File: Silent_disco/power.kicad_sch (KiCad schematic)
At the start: 1 part, among them J1 USB_B_Micro

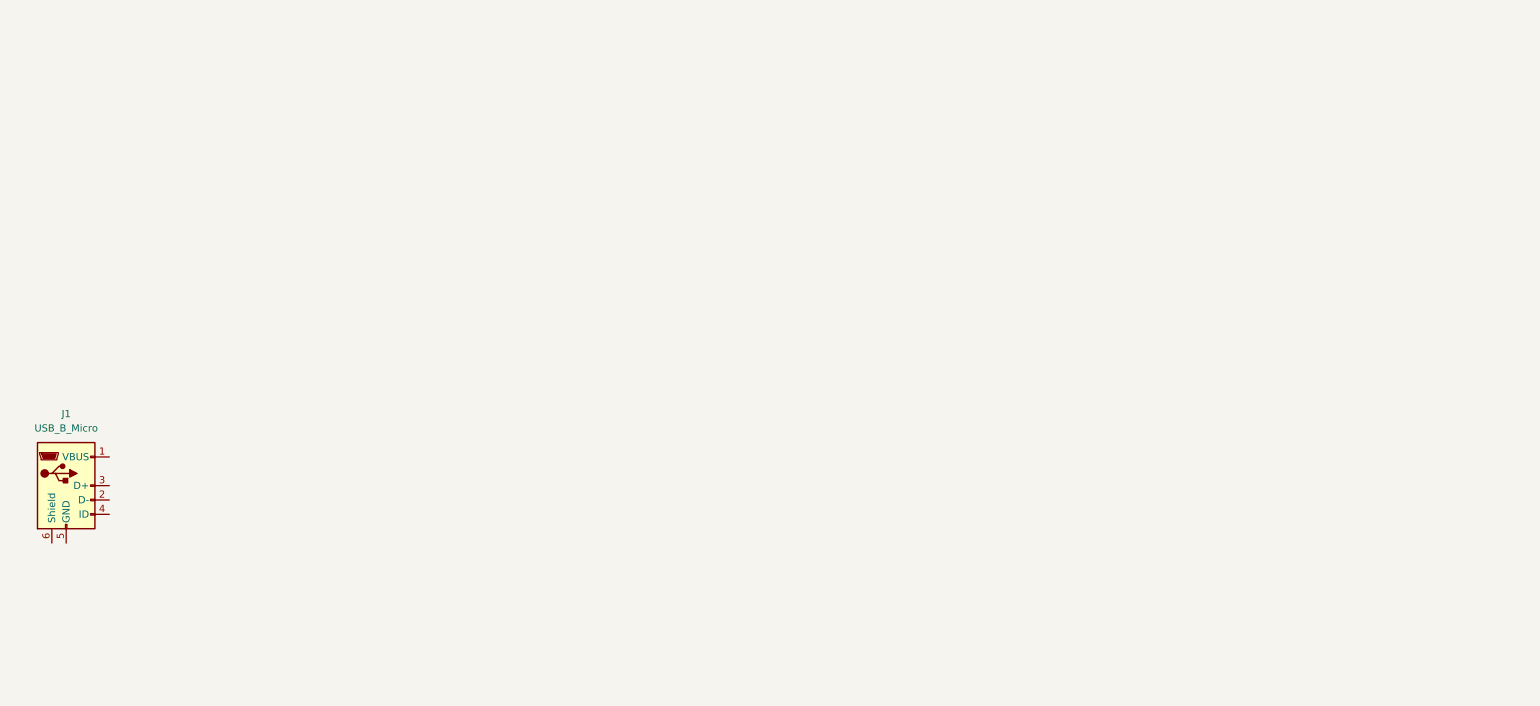
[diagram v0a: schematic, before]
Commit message: husker ikke hva som ble endret her
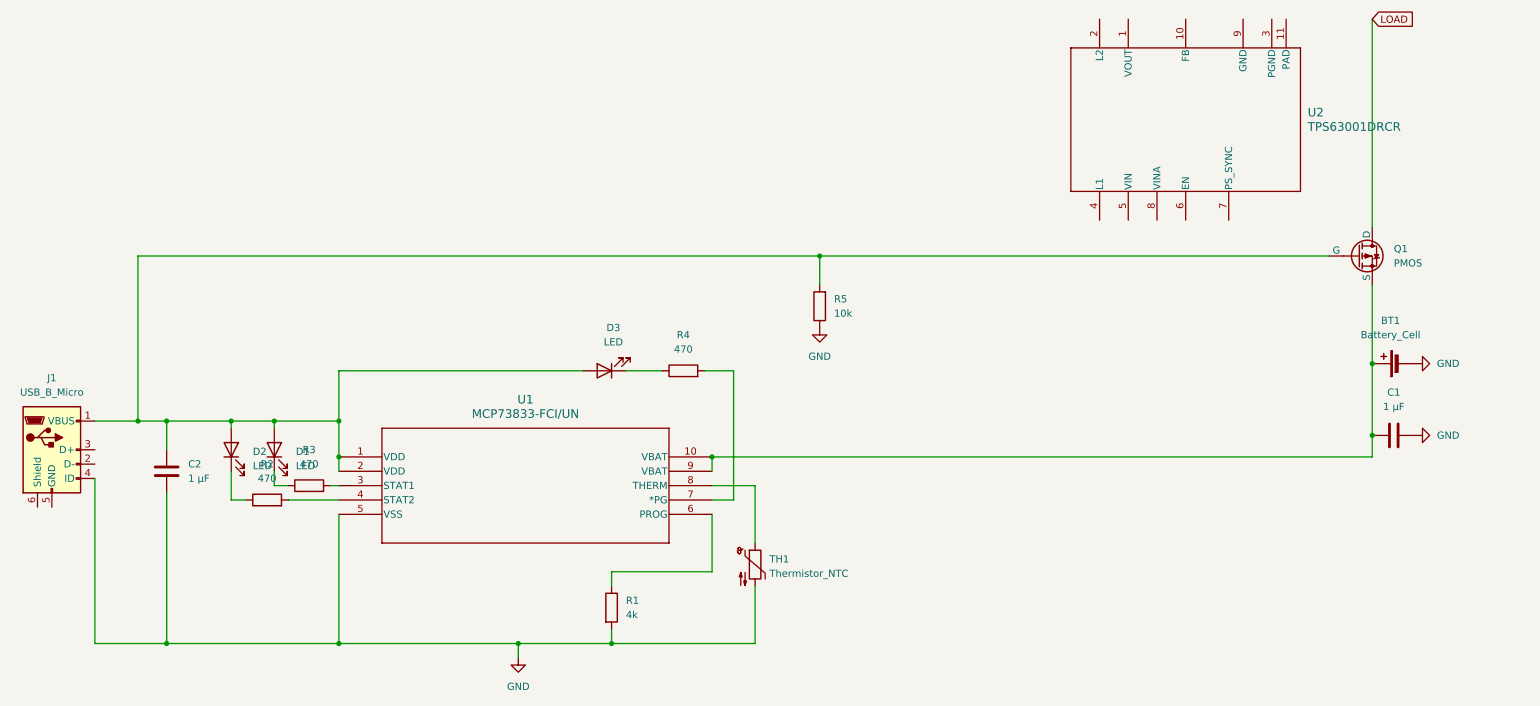
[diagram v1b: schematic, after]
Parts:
- added BT1: Battery_Cell, symbol Device:Battery_Cell
- added C1, C2: 1 μF, symbol Device:C
- added D1, D2, D3: LED, symbol Device:LED
- added Q1: PMOS, symbol Simulation_SPICE:PMOS
- added R1: 4k, symbol Device:R
- added R2, R3, R4: 470, symbol Device:R
- added R5: 10k, symbol Device:R
- added TH1: Thermistor_NTC, symbol Device:Thermistor_NTC
- added U1: MCP73833-FCI/UN, MSOP10_MC_MCH, symbol battery_MCP73833:MCP73833-FCI_UN
- added U2: TPS63001DRCR, DRC0010J, symbol TPS63001DRCR:TPS63001DRCR
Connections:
- net at J1.1 (VBUS): now also C2.2, D1.2 (A), D2.2 (A), D3.2 (A), Q1.2 (G), R5.2, U1.1 (VDD), U1.2 (VDD)
- net GND: now reaches J1.4 (ID)
- net GND: now also BT1.2 (-), C1.2, C2.1, R1.2, R5.1, TH1.2, U1.5 (VSS)
- new net: BT1.1 (+), C1.1, Q1.3 (S), U1.10 (VBAT), U1.9 (VBAT)
- new net: R1.1, U1.6 (PROG)
- new net: TH1.1, U1.8 (THERM)
- new net: R3.2, U1.3 (STAT1)
- new net: R2.2, U1.4 (STAT2)
- new net: R4.2, U1.7 (*PG)
- new net: D1.1 (K), R3.1
- new net: D2.1 (K), R2.1
- new net: D3.1 (K), R4.1
- new net LOAD: Q1.1 (D)
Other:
- moved on the sheet: J1

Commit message: add stuff
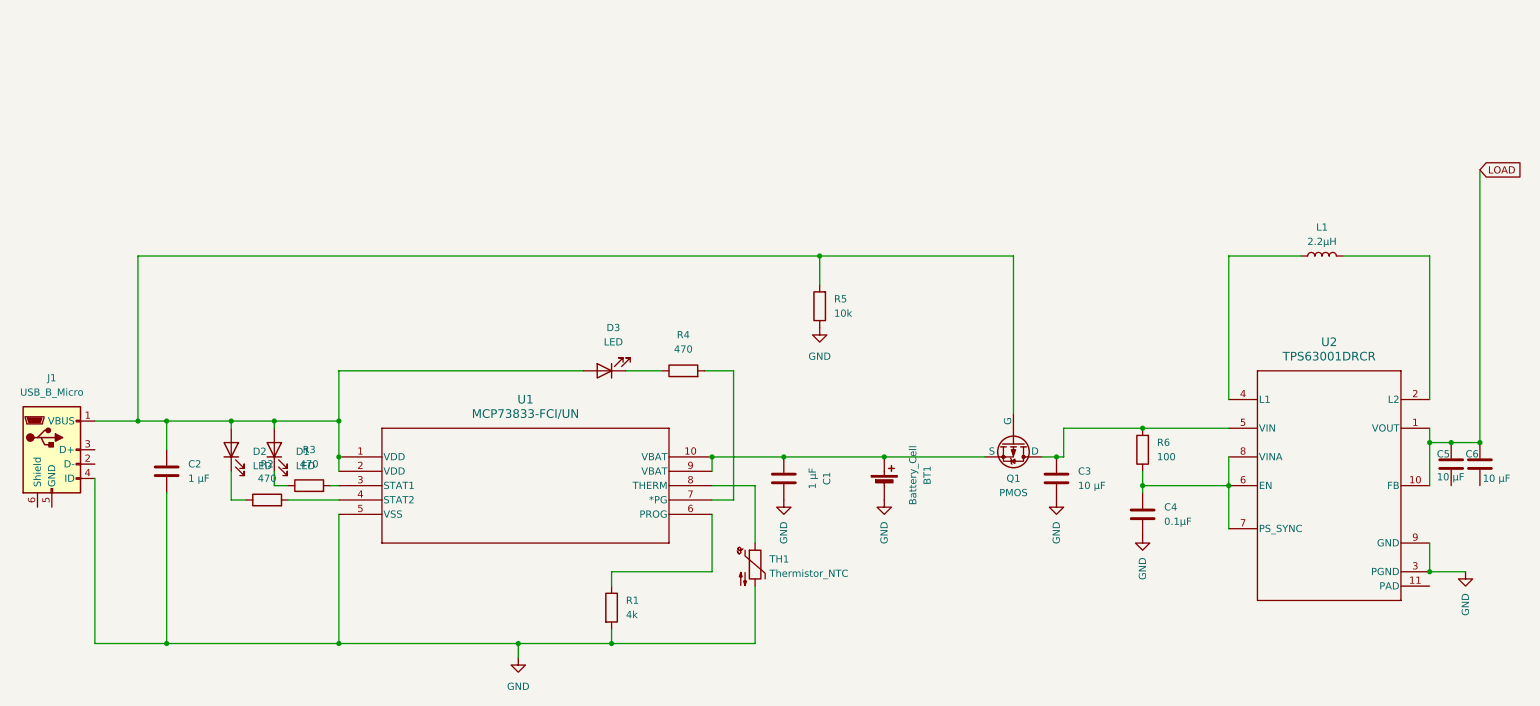
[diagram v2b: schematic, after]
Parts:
- added C3, C5, C6: 10 μF, symbol Device:C
- added C4: 0.1μF, symbol Device:C
- added L1: 2.2μH, symbol Device:L
- added R6: 100, symbol Device:R
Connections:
- net GND: now also U2.3 (PGND), U2.9 (GND), C3.2, C4.2
- net LOAD: now also U2.1 (VOUT), U2.10 (FB), C5.1, C6.1; no longer Q1.1 (D)
- net at U2.2 (L2): now also L1.2
- net at U2.4 (L1): now also L1.1
- net at U2.5 (VIN): now also Q1.1 (D), C3.1, R6.2
- net at U2.6 (EN): now also U2.7 (PS_SYNC), U2.8 (VINA), C4.1, R6.1
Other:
- moved on the sheet: BT1, C1, Q1, U2
